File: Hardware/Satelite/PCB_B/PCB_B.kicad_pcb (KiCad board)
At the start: 2 copper layers, 54 x 54 mm, 66 parts, among them IC1 MCP1642B-50I_MS, IC2 MCP1642B-50I_MS, J1 Conector_PCB_B-C, J2 Conector_PCB_A-B, U1 MIC5323-3.3YD5_TR, U2 ADP2108AUJ-3.3, U3 INA194, U4 MCP6001-OT, U5 INA194, U6 MCP6001-OT, U7 INA194, U8 BQ24091DGQT, U9 BQ27441DRZR-G1A

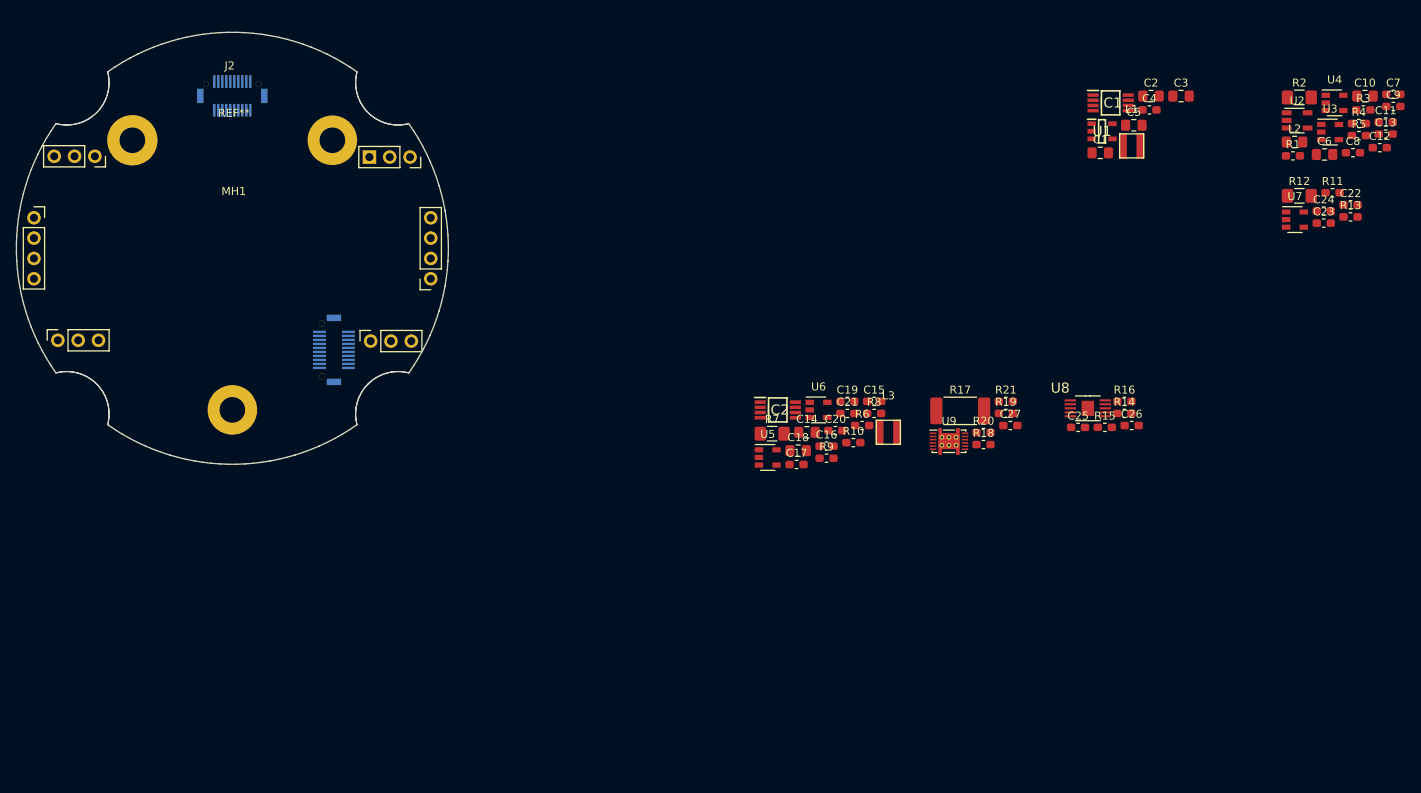
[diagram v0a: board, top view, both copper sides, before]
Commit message: PCB B WIP
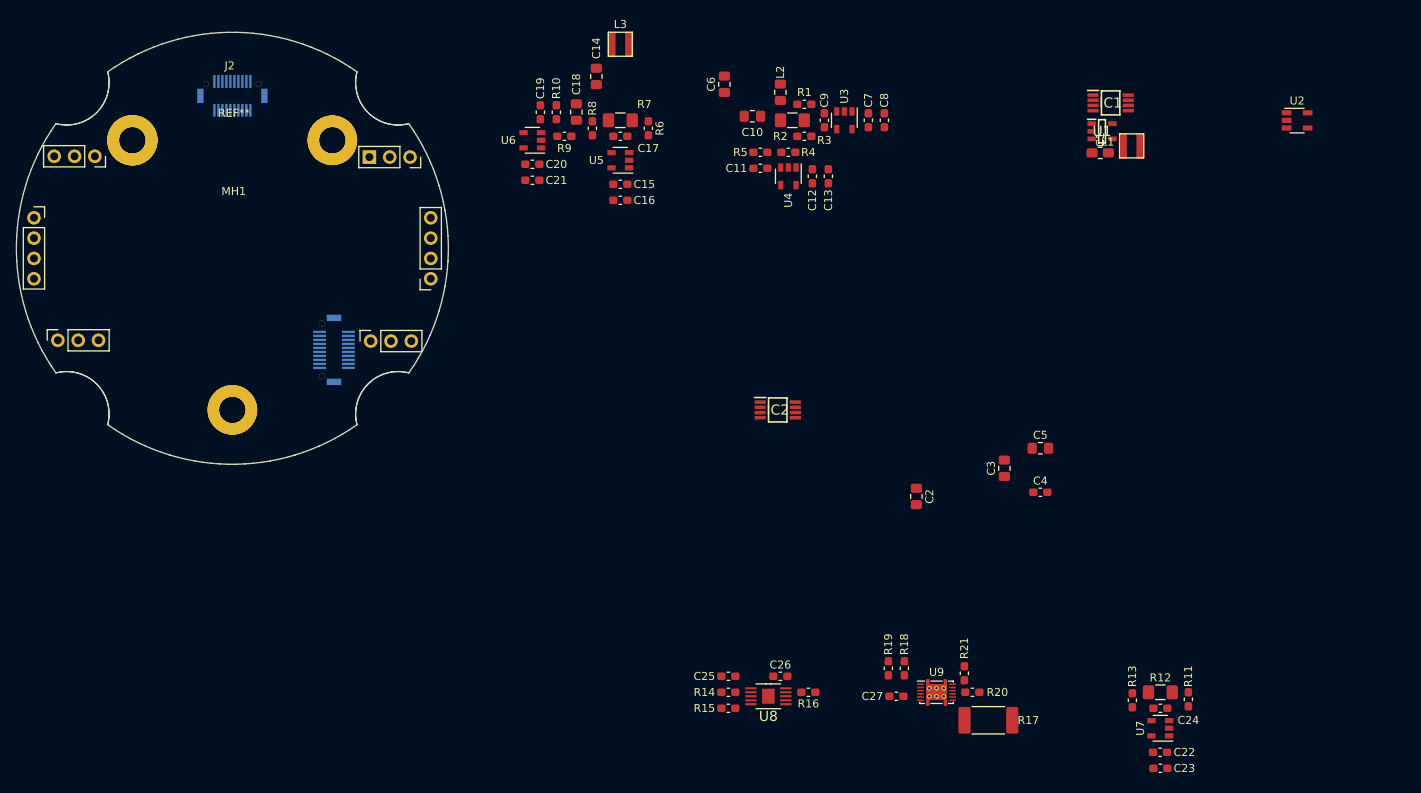
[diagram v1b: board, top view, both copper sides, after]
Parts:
- added MH1: MH_CanSat, AXTEC:MH_CanSat, F.Cu at (0.00, 0.00)
- moved C11 78.4 mm to (66.0, -10.0)
- moved C10 76.6 mm to (65.0, -16.5)
- moved C6 75.5 mm to (61.5, -20.5), turned to 90 degrees
- moved R5 74.8 mm to (66.0, -12.0)
- moved C22 72.5 mm to (116.0, 63.0), turned to 180 degrees
- moved R4 71.4 mm to (69.5, -12.0)
- moved C9 71.1 mm to (74.0, -16.0), turned to 90 degrees
- moved C23 71.1 mm to (116.0, 65.0), turned to 180 degrees
- moved C12 71.0 mm to (72.5, -9.00), turned to 270 degrees
- moved R3 70.0 mm to (71.5, -14.0)
- moved C13 69.9 mm to (74.5, -9.00), turned to 270 degrees
- moved U4 68.9 mm to (69.5, -9.00), turned to 270 degrees
- moved R13 66.3 mm to (112.5, 56.5), turned to 90 degrees
- moved R11 65.8 mm to (119.5, 56.4), turned to 90 degrees
- moved U7 65.8 mm to (116.0, 60.0), turned to 180 degrees
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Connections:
- C10 pad 2: +3V3 -> Net-(C10-Pad2)
- L2 pad 2: Net-(L2-Pad2) -> Net-(C10-Pad2)
- R1 pad 1: Net-(L2-Pad2) -> Net-(C10-Pad2)
- R17 pad 2: /Fuel Gauge/VBAT -> /Sensado Corriente/OUT
- R2 pad 2: Net-(L2-Pad2) -> Net-(C10-Pad2)
- U2 pad 4: +3V3 -> Net-(C10-Pad2)
- U9 pad 6: /Fuel Gauge/VBAT -> /Sensado Corriente/OUT
- U9 pad 8: /Fuel Gauge/VBAT -> /Sensado Corriente/OUT

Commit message: Revert "PCB B WIP"
This reverts commit 7e9720afefe395d959b0157ab5be25ebb8bd8a98.
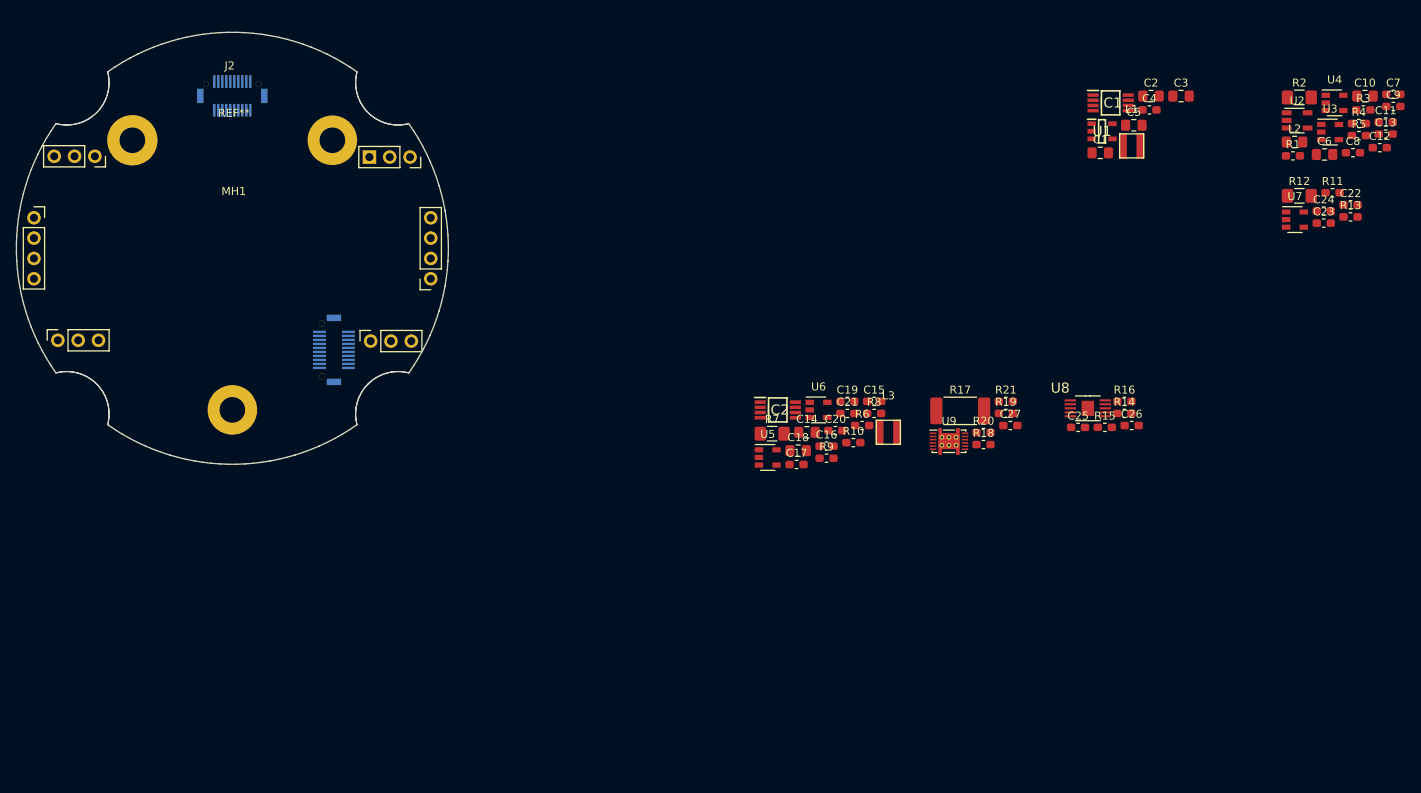
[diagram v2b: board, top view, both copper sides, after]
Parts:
- removed the MH1 at (0.00, 0.00)
- moved C11 78.4 mm to (144.2, -15.8)
- moved C10 76.6 mm to (141.6, -19.0)
- moved C6 75.5 mm to (136.5, -11.7), turned to 0 degrees
- moved R5 74.8 mm to (140.8, -14.1)
- moved C22 72.5 mm to (139.8, -5.43), turned to 0 degrees
- moved R4 71.4 mm to (140.8, -15.6)
- moved C9 71.1 mm to (145.1, -17.7), turned to 0 degrees
- moved C23 71.1 mm to (136.4, -3.14), turned to 0 degrees
- moved C12 71.0 mm to (143.4, -12.6), turned to 0 degrees
- moved R3 70.0 mm to (141.4, -17.3)
- moved C13 69.9 mm to (144.2, -14.3), turned to 0 degrees
- moved U4 68.9 mm to (137.8, -18.2), turned to 0 degrees
- moved R13 66.3 mm to (139.8, -3.92), turned to 0 degrees
- moved R11 65.8 mm to (137.5, -6.94), turned to 0 degrees
- moved U7 65.8 mm to (132.8, -3.58), turned to 0 degrees
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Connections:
- C10 pad 2: Net-(C10-Pad2) -> +3V3
- L2 pad 2: Net-(C10-Pad2) -> Net-(L2-Pad2)
- R1 pad 1: Net-(C10-Pad2) -> Net-(L2-Pad2)
- R17 pad 2: /Sensado Corriente/OUT -> /Fuel Gauge/VBAT
- R2 pad 2: Net-(C10-Pad2) -> Net-(L2-Pad2)
- U2 pad 4: Net-(C10-Pad2) -> +3V3
- U9 pad 6: /Sensado Corriente/OUT -> /Fuel Gauge/VBAT
- U9 pad 8: /Sensado Corriente/OUT -> /Fuel Gauge/VBAT
